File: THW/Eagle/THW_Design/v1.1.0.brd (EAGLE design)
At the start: 73.5 x 175.6 mm, 46 parts, among them U1 ADA4091-2ARZ-RL

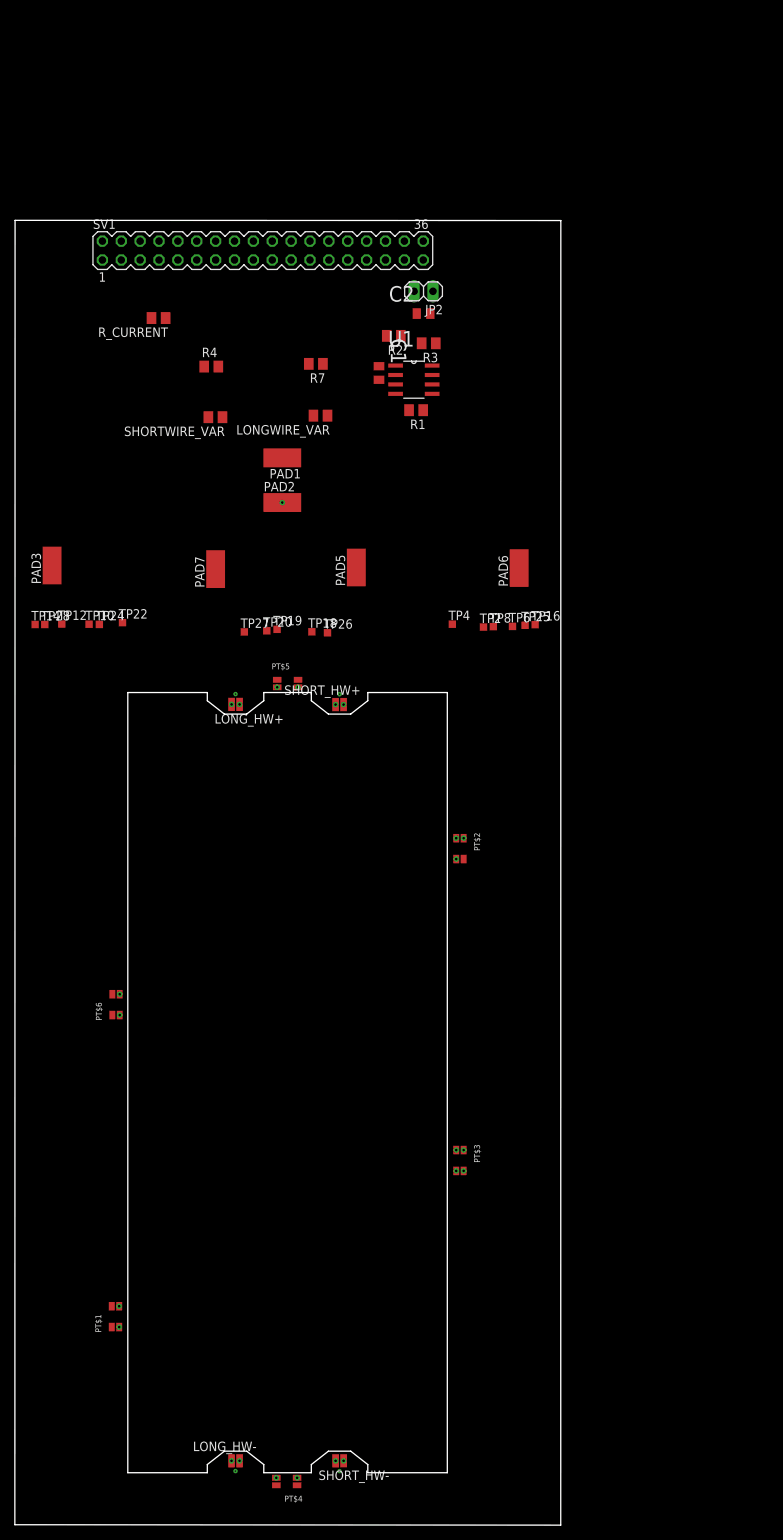
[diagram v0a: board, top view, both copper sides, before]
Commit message: routing
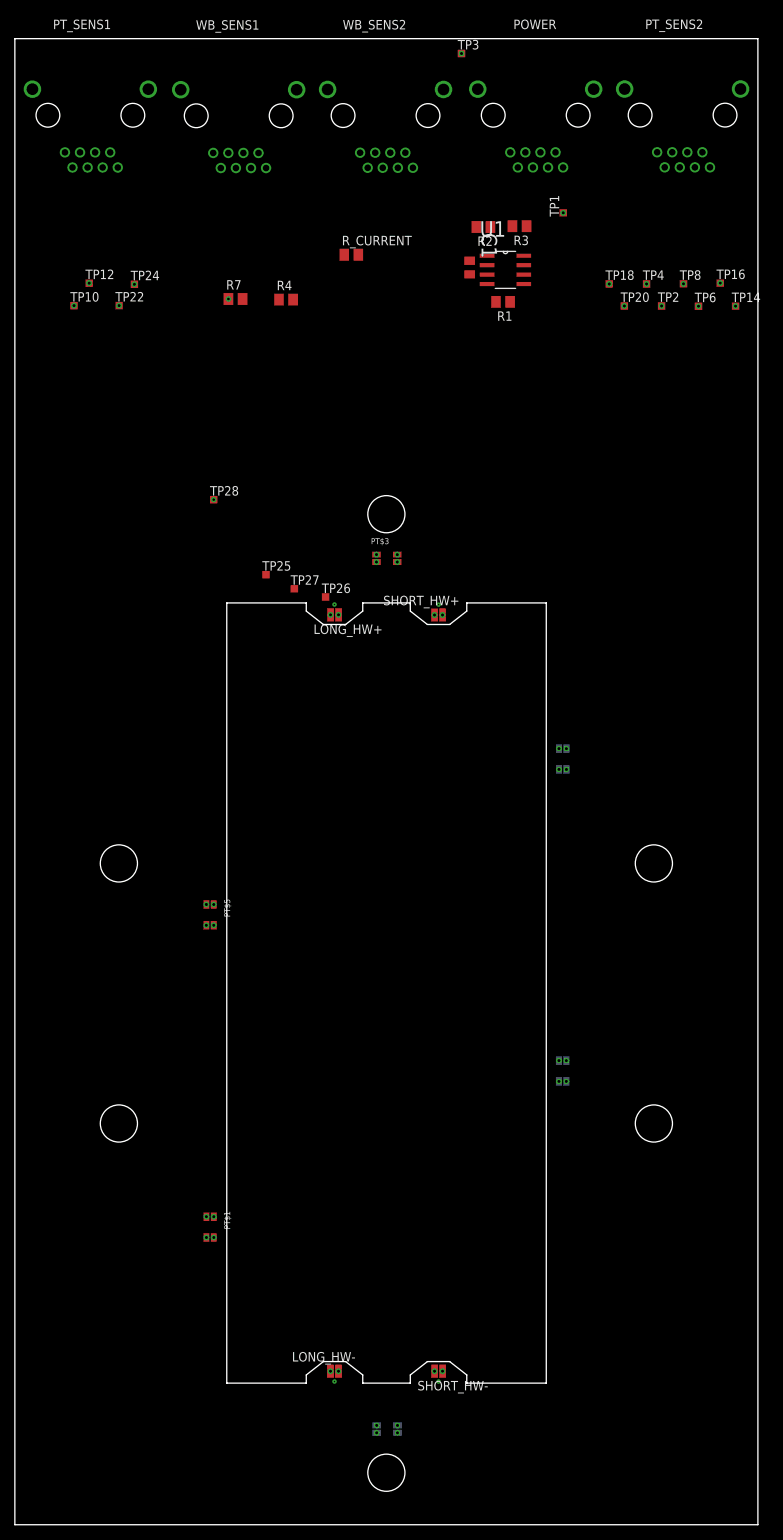
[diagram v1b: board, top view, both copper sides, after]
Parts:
- removed C2: 0805YC103J4T2A, 0805YC103J4T2A:CAPC2012X94N
- removed JP2: (no value), pinhead:1X02
- removed LONGWIRE_VAR, SHORTWIRE_VAR: (no value), resistor:M0805
- removed PAD1, PAD2, PAD3, PAD5, PAD6, PAD7: (no value), wirepad:SMD2,54-5,08
- removed PT$6: PTS1206A, PTS1206:CAPMP3216X166
- removed SV1: (no value), con-lstb:MA18-2
- removed TP19: TPTP10SQ, testpad:TP10SQ
- added POWER, PT_SENS1, PT_SENS2, WB_SENS1, WB_SENS2: RJ45_CONNECTOR, RJ45_CONNECTOR:RJ45_CONNNECTOR
- added PT$0: PTS1206A, PTS1206:CAPMP3216X166
- added TP1, TP3: TPTP10SQ, testpad:TP10SQ
- moved TP14 103.5 mm to (97.0, 164.0)
- moved PT$3 81.6 mm to (50.1, 130.1), turned to 0 degrees
- moved TP20 65.0 mm to (82.0, 164.0)
- moved TP18 61.6 mm to (80.0, 167.0)
- moved TP8 52.8 mm to (90.0, 167.0)
- moved TP4 52.7 mm to (85.0, 167.0)
- moved TP16 52.3 mm to (94.9, 167.1)
- moved TP6 49.8 mm to (92.0, 164.0)
- moved TP2 49.4 mm to (87.0, 164.0)
- moved TP12 46.0 mm to (10.0, 167.1)
- moved TP24 46.0 mm to (16.1, 166.9)
- moved TP10 42.9 mm to (7.97, 164.1)
- moved TP22 42.7 mm to (14.0, 164.1)
- moved TP25 35.5 mm to (33.8, 127.9)
- moved PT$2 33.0 mm to (73.7, 61.1), flipped to the bottom
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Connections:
- removed net B$2: PT$1.-
- removed net LONG_HW_SENS+: LONG_HW+.P$2, TP27.TP
- removed net PT+: PAD1.1, PT$1.+, PT$2.+, PT$3.+, PT$4.+, PT$5.+, PT$6.+
- removed net PT-: PAD2.1, PT$2.-, PT$3.-, PT$4.-, PT$5.-, PT$6.-
- removed net PT6_S+: PT$6.SENS+, TP22.TP
- removed net PT6_S-: PT$6.SENS-, TP24.TP
- new net PT0_S+: PT$0.SENS+, PT_SENS2.3, TP2.TP
- new net PT0_S-: PT$0.SENS-, PT_SENS2.4, TP4.TP
- new net PT_CURRENT+: POWER.7, PT$0.+, PT$0.-, PT$1.+, PT$1.-, PT$2.+, PT$2.-, PT$3.+, PT$3.-, PT$4.+, PT$4.-, PT$5.+, TP1.TP
- new net PT_CURRENT-: POWER.8, PT$5.-, TP3.TP
- new net WB_CURRENT+: POWER.3, R_CURRENT.1, WB_SENS2.1
- new net WB_CURRENT-: LONG_HW-.P$2, POWER.4, R7.1, WB_SENS2.6
- net GND: now also POWER.6, WB_SENS2.8; no longer C2.2, JP2.1, LONGWIRE_VAR.2, R7.1, SV1.25, SV1.4
- net LONG_HW+: no longer LONG_HW+.P$1, PAD7.1, SHORTWIRE_VAR.1, SV1.24, SV1.27
- net LONG_HW-: no longer LONGWIRE_VAR.1, LONG_HW-.P$2, PAD3.1, SV1.26
- net LONG_HW_SENS-: now also WB_SENS1.2
- net OPAMP_OUTPUT: now also WB_SENS2.7; no longer SV1.3
- net PT1_S+: now also PT$1.SENS+, PT_SENS1.2, TP10.TP; no longer PT$2.SENS+, TP2.TP
- net PT1_S-: now also PT$1.SENS-, PT_SENS1.1, TP12.TP; no longer PT$2.SENS-, TP4.TP
- net PT2_S+: now also PT$2.SENS+, PT_SENS2.5; no longer PT$3.SENS+
- net PT2_S-: now also PT$2.SENS-, PT_SENS2.6; no longer PT$3.SENS-
- net PT3_S+: now also PT$3.SENS+, PT_SENS2.2, TP18.TP; no longer PT$1.SENS+, TP10.TP
- net PT3_S-: now also PT$3.SENS-, PT_SENS2.1, TP20.TP; no longer PT$1.SENS-, TP12.TP
- net PT4_S+: now also PT_SENS2.8
- net PT4_S-: now also PT_SENS2.7
- net PT5_S+: now also PT_SENS1.4, TP22.TP; no longer TP18.TP
- net PT5_S-: now also PT_SENS1.3, TP24.TP; no longer TP20.TP
- net SHORT_HW+: now also WB_SENS2.2, WB_SENS2.3; no longer PAD5.1, SV1.30
- net SHORT_HW-: now also LONG_HW+.P$1; no longer PAD6.1, SHORTWIRE_VAR.2, SV1.28
- net SHORT_HW_SENS+: now also WB_SENS1.8
- net SHORT_HW_SENS-: now also LONG_HW+.P$2, TP27.TP, WB_SENS1.1, WB_SENS1.5, WB_SENS1.7
- net SUMMING_OP_AMP: now also WB_SENS1.6, WB_SENS2.4, WB_SENS2.5; no longer SV1.23
- net VSS: now also POWER.5; no longer C2.1, JP2.2, R_CURRENT.1, SV1.29
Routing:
- net PT_CURRENT+: track 0.00 -> 330.4 mm, vias 0 -> 12
- net PT_CURRENT-: track 0.00 -> 212.6 mm, vias 0 -> 2
- net WB_CURRENT-: track 0.00 -> 162.3 mm, vias 0 -> 2
- net PT-: track 149.4 -> 0.00 mm, vias 3 -> 0
- net LONG_HW-: track 138.5 -> 0.00 mm, vias 1 -> 0
- net PT1_S-: track 26.8 -> 153.9 mm, vias 1 -> 2
- net PT1_S+: track 34.2 -> 159.7 mm, vias 1 -> 2
- net PT5_S+: track 8.01 -> 114.2 mm, vias 1 -> 2
- net PT5_S-: track 7.43 -> 108.6 mm, vias 1 -> 2
- net PT0_S+: track 0.00 -> 90.8 mm, vias 0 -> 2
- net PT0_S-: track 0.00 -> 88.3 mm, vias 0 -> 2
- net PT4_S+: track 149.6 -> 214.6 mm, vias 1 -> 2
- net PT2_S-: track 71.9 -> 132.3 mm, vias 1 -> 2
- net PT4_S-: track 148.4 -> 206.7 mm, vias 1 -> 2
- net PT6_S-: track 55.8 -> 0.00 mm, vias 1 -> 0
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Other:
- board size 73.5 x 175.6 mm -> 100 x 200 mm
